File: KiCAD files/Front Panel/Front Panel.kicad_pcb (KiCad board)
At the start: 2 copper layers, 99.1 x 80 mm, 19 parts, among them J1 fixing bolt, J10 led, J11 led, J12 led, J13 led, J14 led, J15 led, J16 led, J17 led, J18 led, J19 led, J2 fixing bolt, J3 fixing bolt, J4 fixing bolt, J5 fixing bolt, J6 fixing bolt, J7 fixing bolt, J8 fixing bolt, J9 reset button

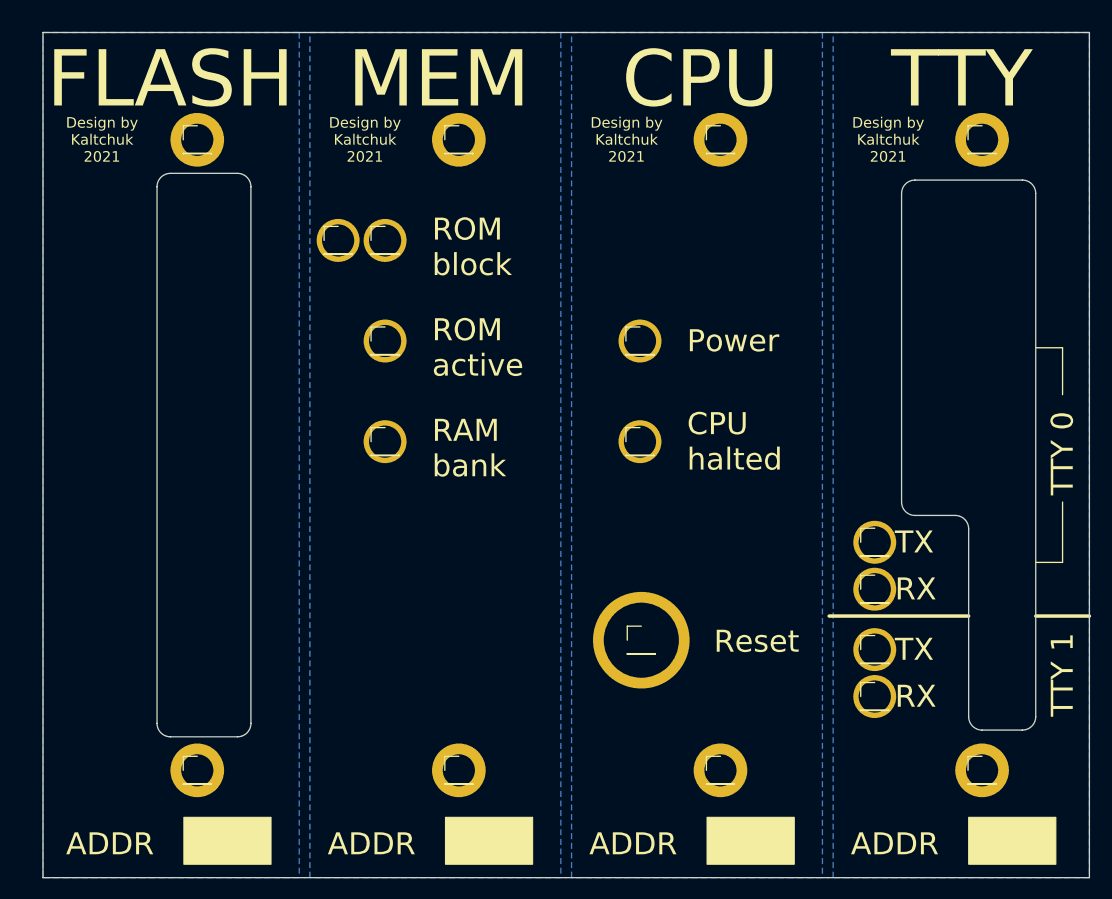
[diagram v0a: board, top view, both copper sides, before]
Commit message: office
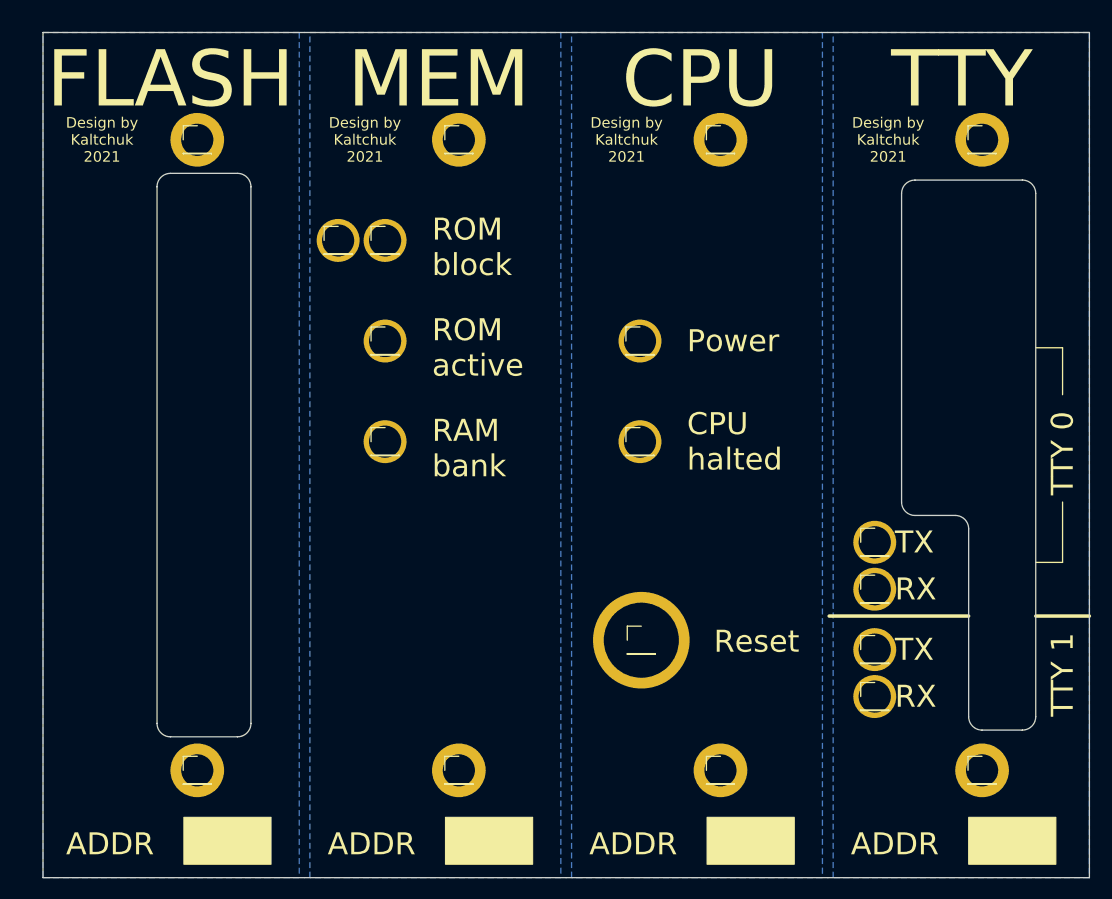
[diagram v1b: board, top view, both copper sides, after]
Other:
- net class Default removed
